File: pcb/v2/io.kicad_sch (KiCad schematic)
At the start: 58 parts, among them J12 Conn_01x04, J13 Conn_01x05, U10 STI9287, U8 TCKE812, U9 CH334R, Y1 12M

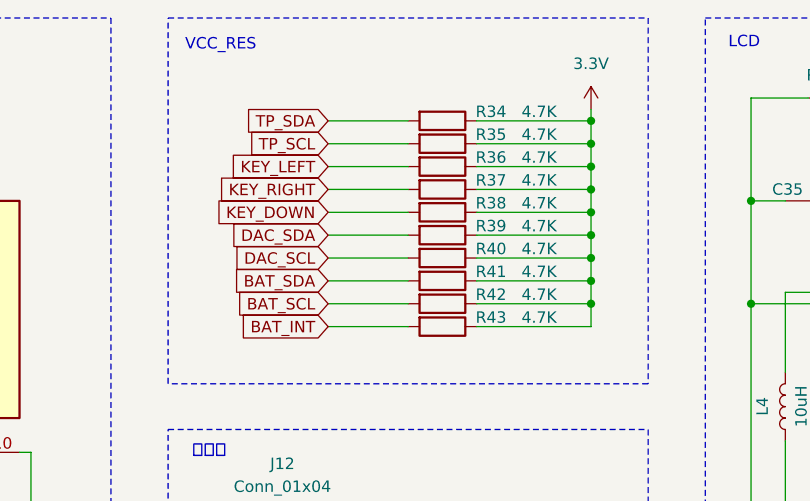
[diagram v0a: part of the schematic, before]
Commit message: up pcb
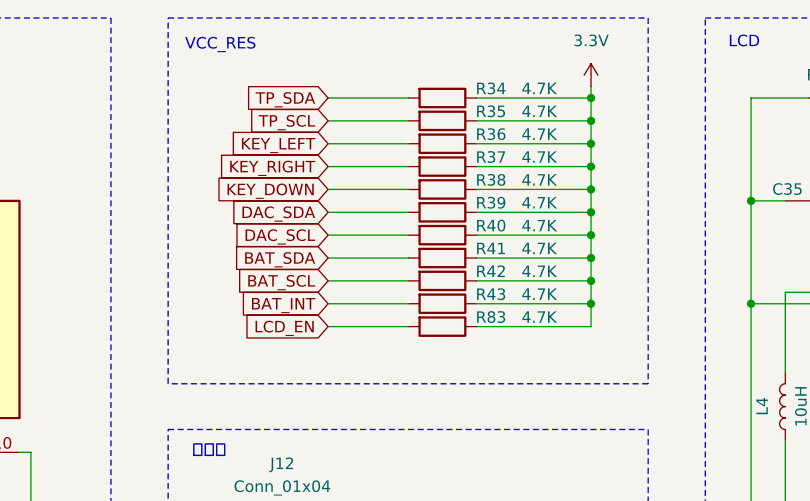
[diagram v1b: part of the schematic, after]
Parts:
- added R83: 4.7K, Capacitor_SMD:C_0402_1005Metric_Pad0.74x0.62mm_HandSolder, symbol Device:R
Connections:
- net 3.3V: now also R83.1
- net LCD_EN: now also R83.2
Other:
- moved on the sheet: R34, R35, R36, R37, R38, R39, R40, R41, R42, R43
